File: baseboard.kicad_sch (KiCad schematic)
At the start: 47 parts, among them J10 AS7265X, J11 TFT_FMC, J12 SERVO1, J13 USER_GPIO, J14 TFT_SPI, J15 SERVO2, J16 FAN, J17 ADC_IN, J18 BME280, J5 POWER, J6 DCMI_CAMERA, J7 LCD_CHAR, J8 UART1, J9 UART2, Q1 BCP56, Q2 BCP56, Q3 BCP56, U2 LM2676S-5, U3 AMS1117-3.3

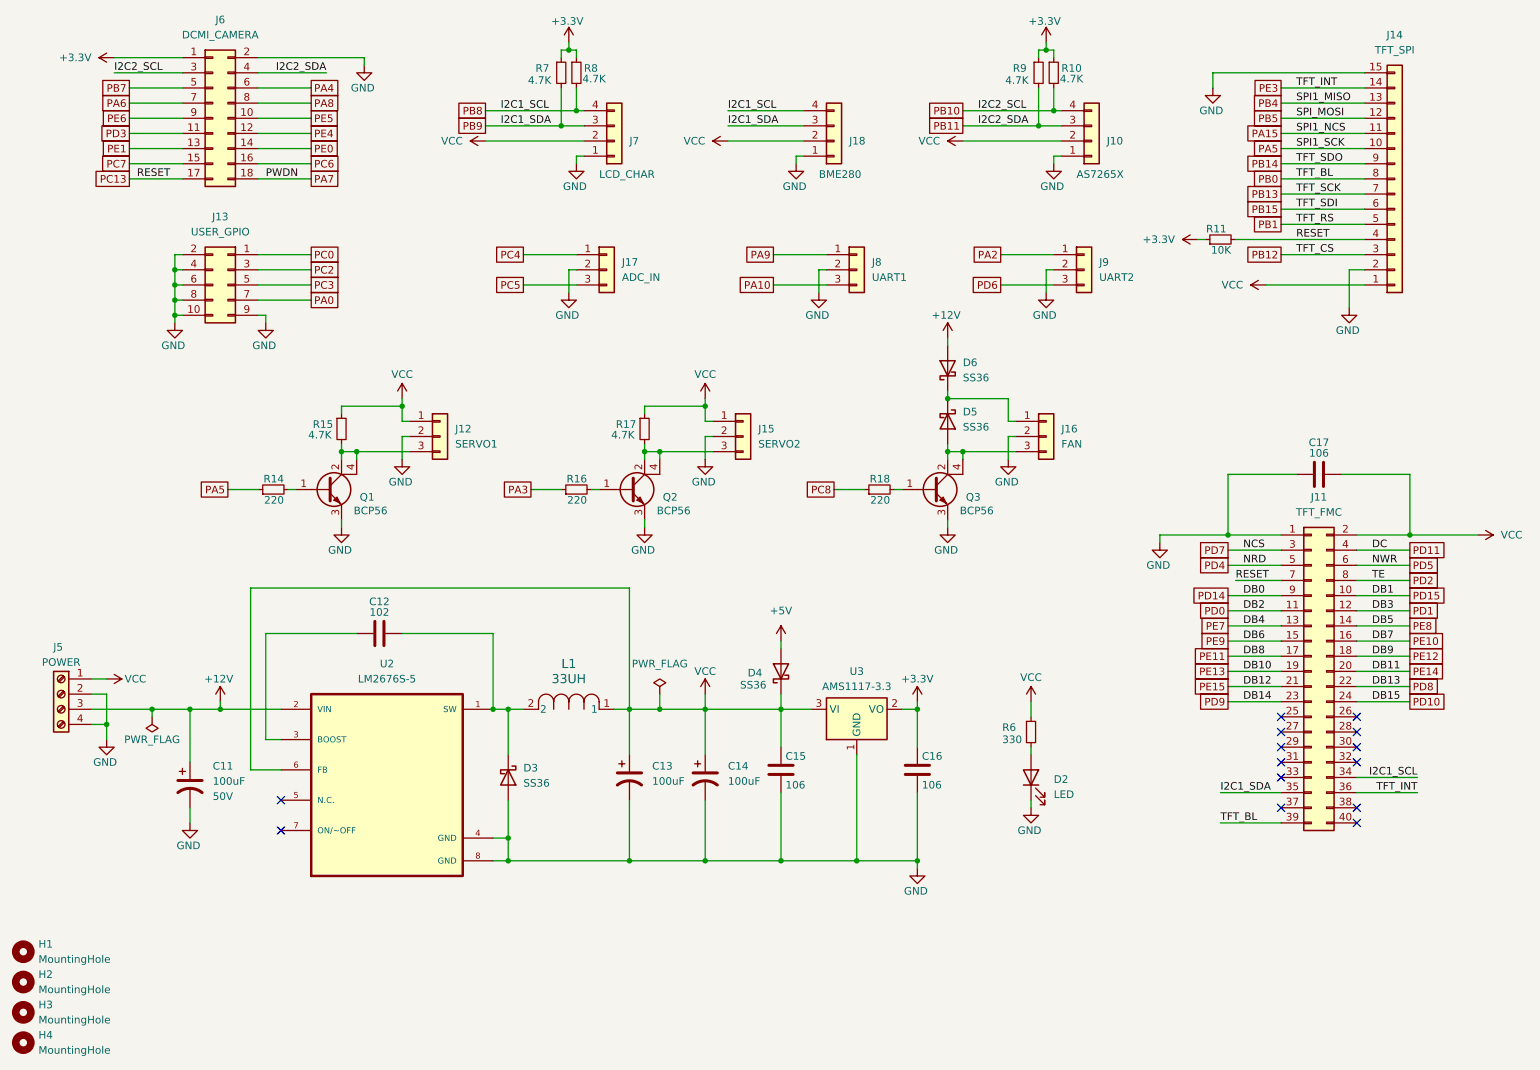
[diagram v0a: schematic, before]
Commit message: snapshot
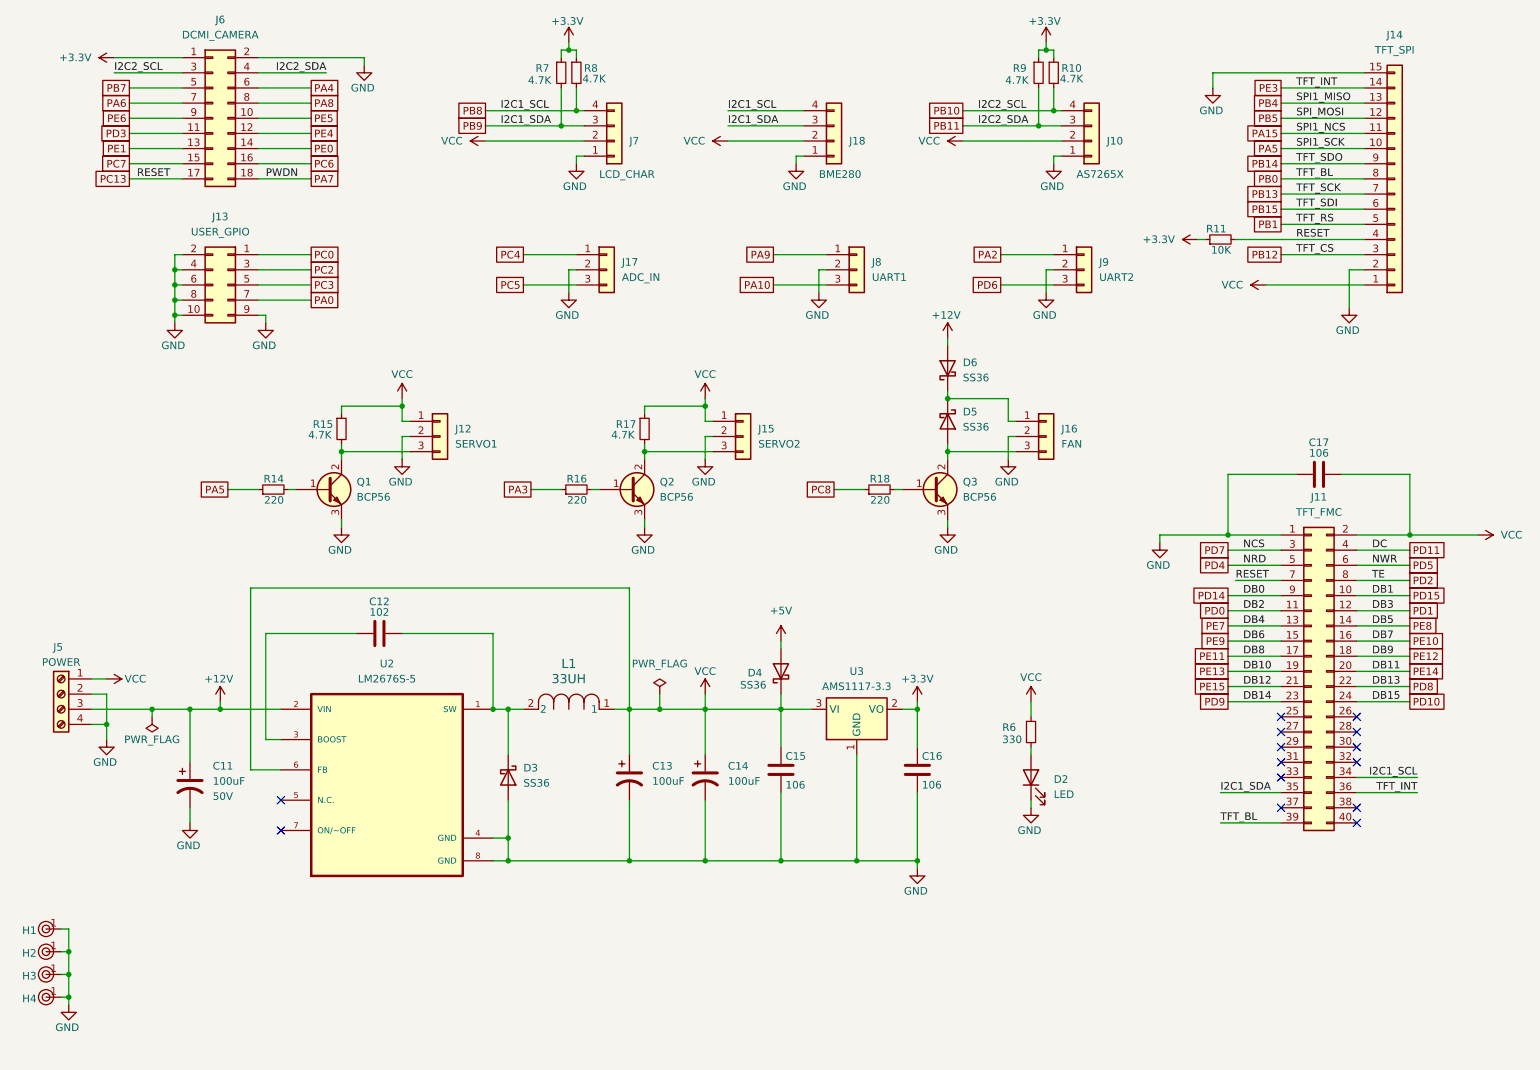
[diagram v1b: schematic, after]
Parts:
- removed H1, H2, H3, H4: MountingHole, MountingHole:MountingHole_3.2mm_M3, symbol LM2676S-3.3_NOPB:MountingHole
- removed Q1, Q2, Q3: BCP56, Package_TO_SOT_SMD:SOT-223-3_TabPin2, symbol Transistor_BJT:BCP56
- added H1, H2, H3, H4: ~, PCM_JLCPCB:Hole, 3mm, symbol PCM_JLCPCB-Manufacturing:Mounting Hole, 3mm, Via Stiched
- added Q1, Q2, Q3: BCP56, PCM_Package_TO_SOT_SMD_AKL:SOT-223-3_TabPin2, symbol PCM_Transistor_BJT_AKL:BCP56
- L1: footprint Inductor_SMD:L_Bourns-SRN8040_8x8.15mm -> JLCPCB:L_SMD,8x8mm
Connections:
- net GND: now also H1.1, H2.1, H3.1, H4.1, Q1.3 (E), Q2.3 (E), Q3.3 (E)
- net at J15.3 (Pin_3), R17.2: now also Q2.2 (C)
- net at D5.2 (A), J16.3 (Pin_3): now also Q3.2 (C)
- net at J12.3 (Pin_3), R15.2: now also Q1.2 (C)
- net at R14.2: now also Q1.1 (B)
- net at R18.2: now also Q3.1 (B)
- net at R16.2: now also Q2.1 (B)
